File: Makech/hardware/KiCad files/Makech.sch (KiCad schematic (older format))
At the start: 49 parts, among them IC1 ULN2803, J1 SWD programmer, J2 USB_B_Micro, J3 ESP32-Exp, SW1 RST, SW2 SW_DPDT_x2, U1 ATSAMD21G18A-AU, U2 CONN_01X04, U3 AP2114_3.3v, X1 Screw_Terminal_1x02

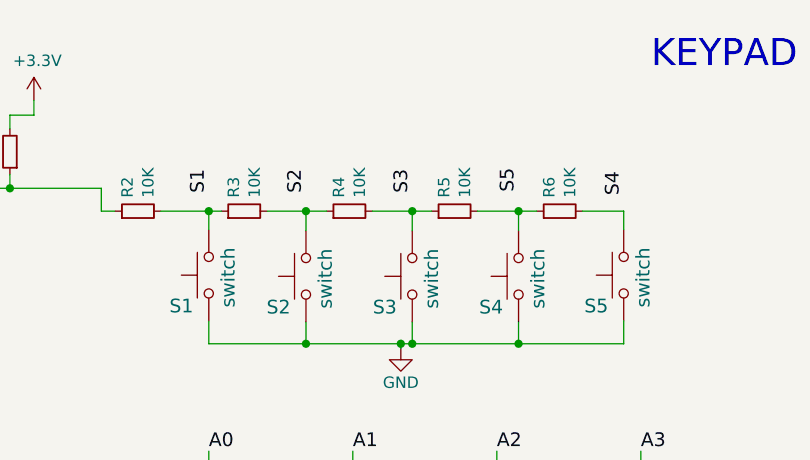
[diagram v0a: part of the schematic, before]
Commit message: Complete
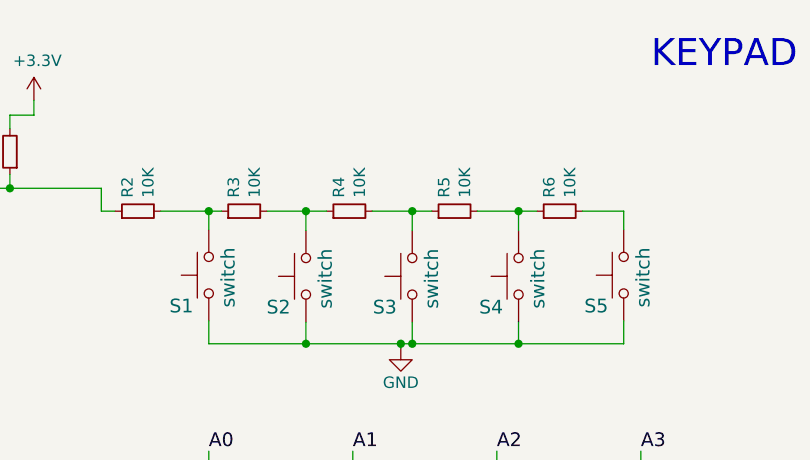
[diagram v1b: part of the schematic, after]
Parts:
- J1: footprint Connector_PinHeader_1.00mm:PinHeader_2x02_P1.00mm_Vertical_SMD -> Connector_PinHeader_2.54mm:PinHeader_2x02_P2.54mm_Vertical_SMD
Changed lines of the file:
@@
 Text Label 7645 2390 0    60   ~ 0
 A3
-Text Label 5755 1260 1    60   ~ 0
-S1
-Text Label 6180 1260 1    60   ~ 0
-S2
-Text Label 6645 1260 1    60   ~ 0
-S3
-Text Label 7110 1255 1    60   ~ 0
-S5
-Text Label 7570 1270 1    60   ~ 0
-S4
 $Comp
 L Makech-rescue:JUMPER--Ogaki-rescue-Makech-rescue-Makech-rescue-Makech-rescue-Makech-rescue-Makech-rescue-Makech-rescue-Makech-rescue-Makech-rescue SJ1
@@
 F 0 "J1" H 1305 5897 50  0000 C CNN
 F 1 "SWD programmer" H 1305 5806 50  0000 C CNN
-F 2 "Connector_PinHeader_1.00mm:PinHeader_2x02_P1.00mm_Vertical_SMD" H 1255 5680 50  0001 C CNN
+F 2 "Connector_PinHeader_2.54mm:PinHeader_2x02_P2.54mm_Vertical_SMD" H 1255 5680 50  0001 C CNN
 F 3 "~" H 1255 5680 50  0001 C CNN
 	1    1255 5680
